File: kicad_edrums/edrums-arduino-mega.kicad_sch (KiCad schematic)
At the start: 24 parts, among them J1 midi out, P1 piezo, P2 piezo, P3 piezo, P4 piezo

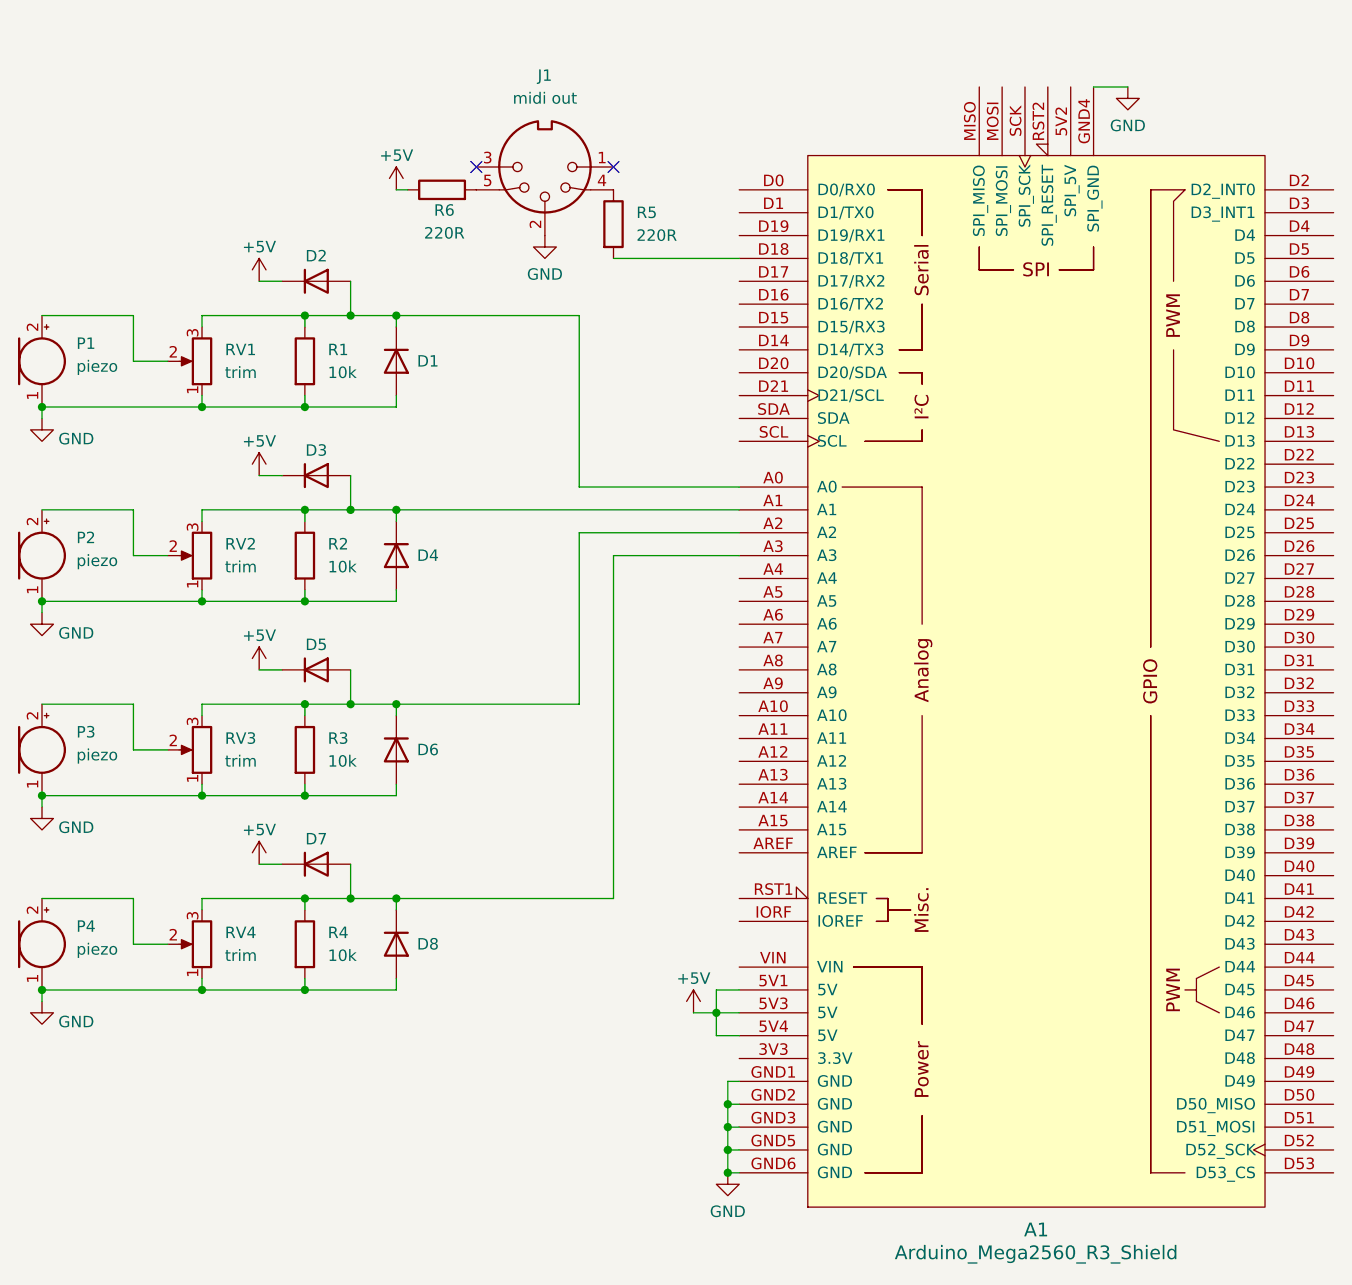
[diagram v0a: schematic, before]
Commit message: schematic
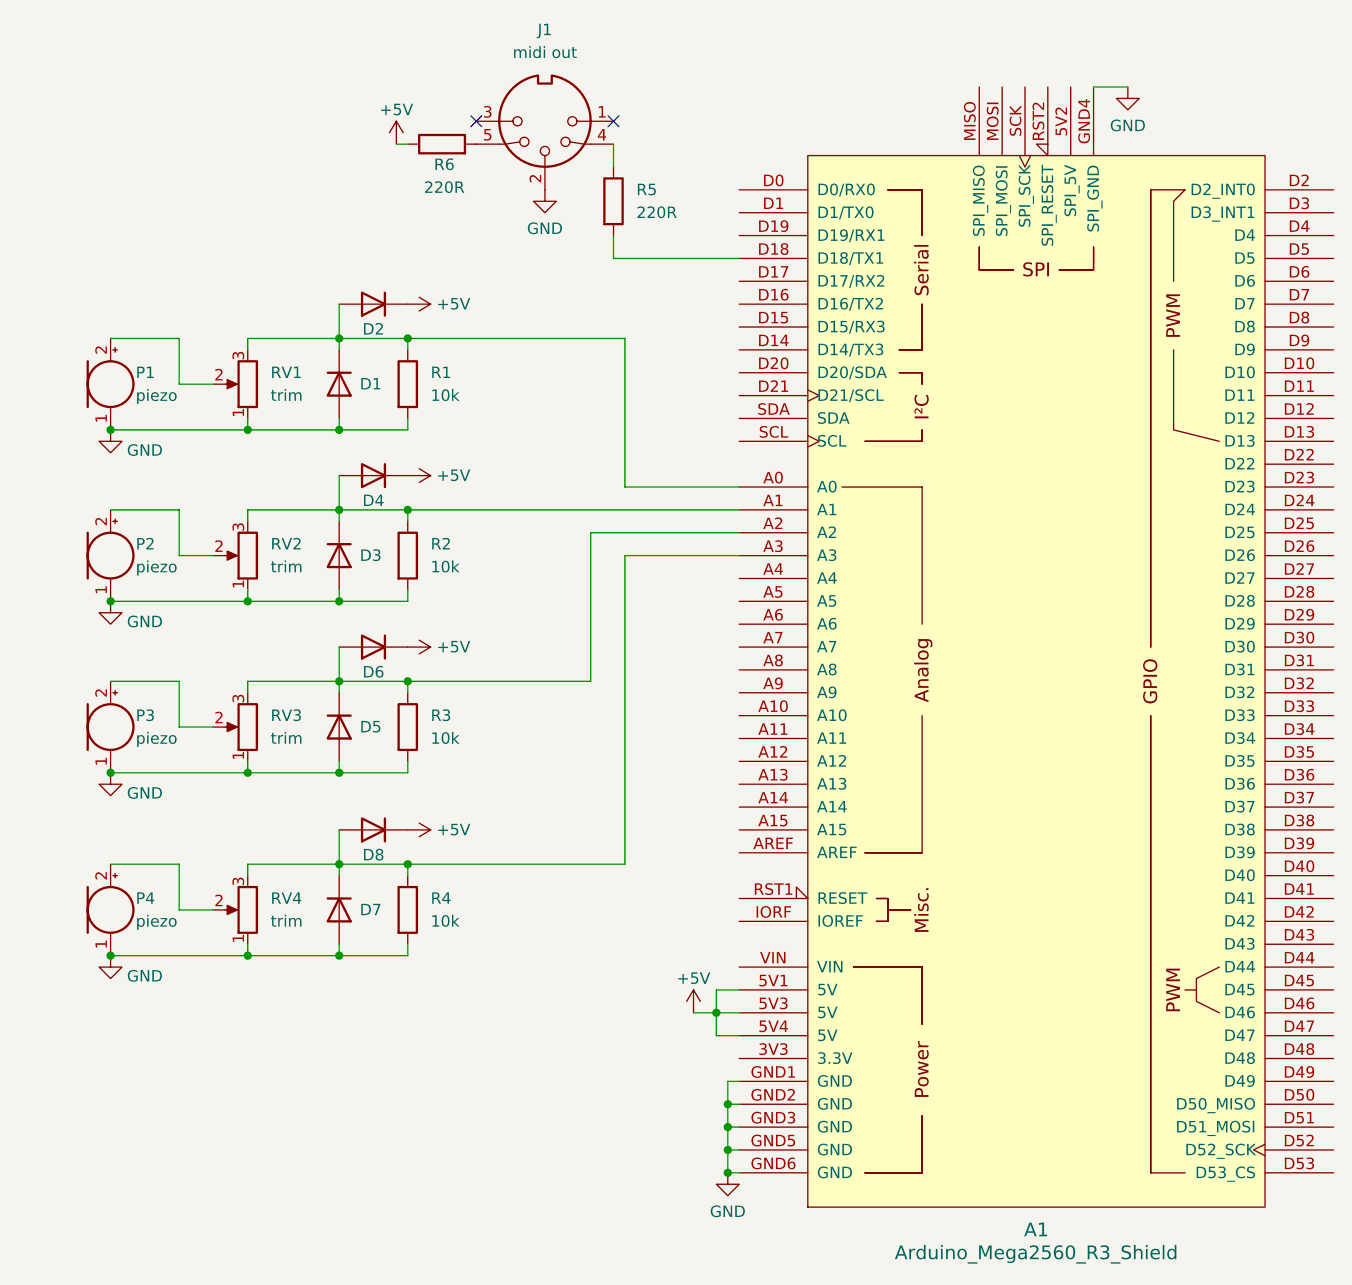
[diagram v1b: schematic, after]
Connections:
- net +5V: now also D4.1 (K), D6.1 (K), D8.1 (K); no longer D3.1 (K), D5.1 (K), D7.1 (K)
- net GND: now also D3.2 (A), D5.2 (A), D7.2 (A); no longer D4.2 (A), D6.2 (A), D8.2 (A)
- net at A1.A1, R2.1, RV2.3: now also D3.1 (K), D4.2 (A); no longer D3.2 (A), D4.1 (K)
- net at A1.A2, R3.1, RV3.3: now also D5.1 (K), D6.2 (A); no longer D5.2 (A), D6.1 (K)
- net at A1.A3, R4.1, RV4.3: now also D7.1 (K), D8.2 (A); no longer D7.2 (A), D8.1 (K)
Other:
- moved on the sheet: D1, D2, J1, P1, R1, R5, R6, RV1
